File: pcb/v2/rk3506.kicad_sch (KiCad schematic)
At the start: 15 parts, among them J1 Conn_01x02, J2 Conn_01x03, J3 Conn_01x02, U1 SOM3562_18

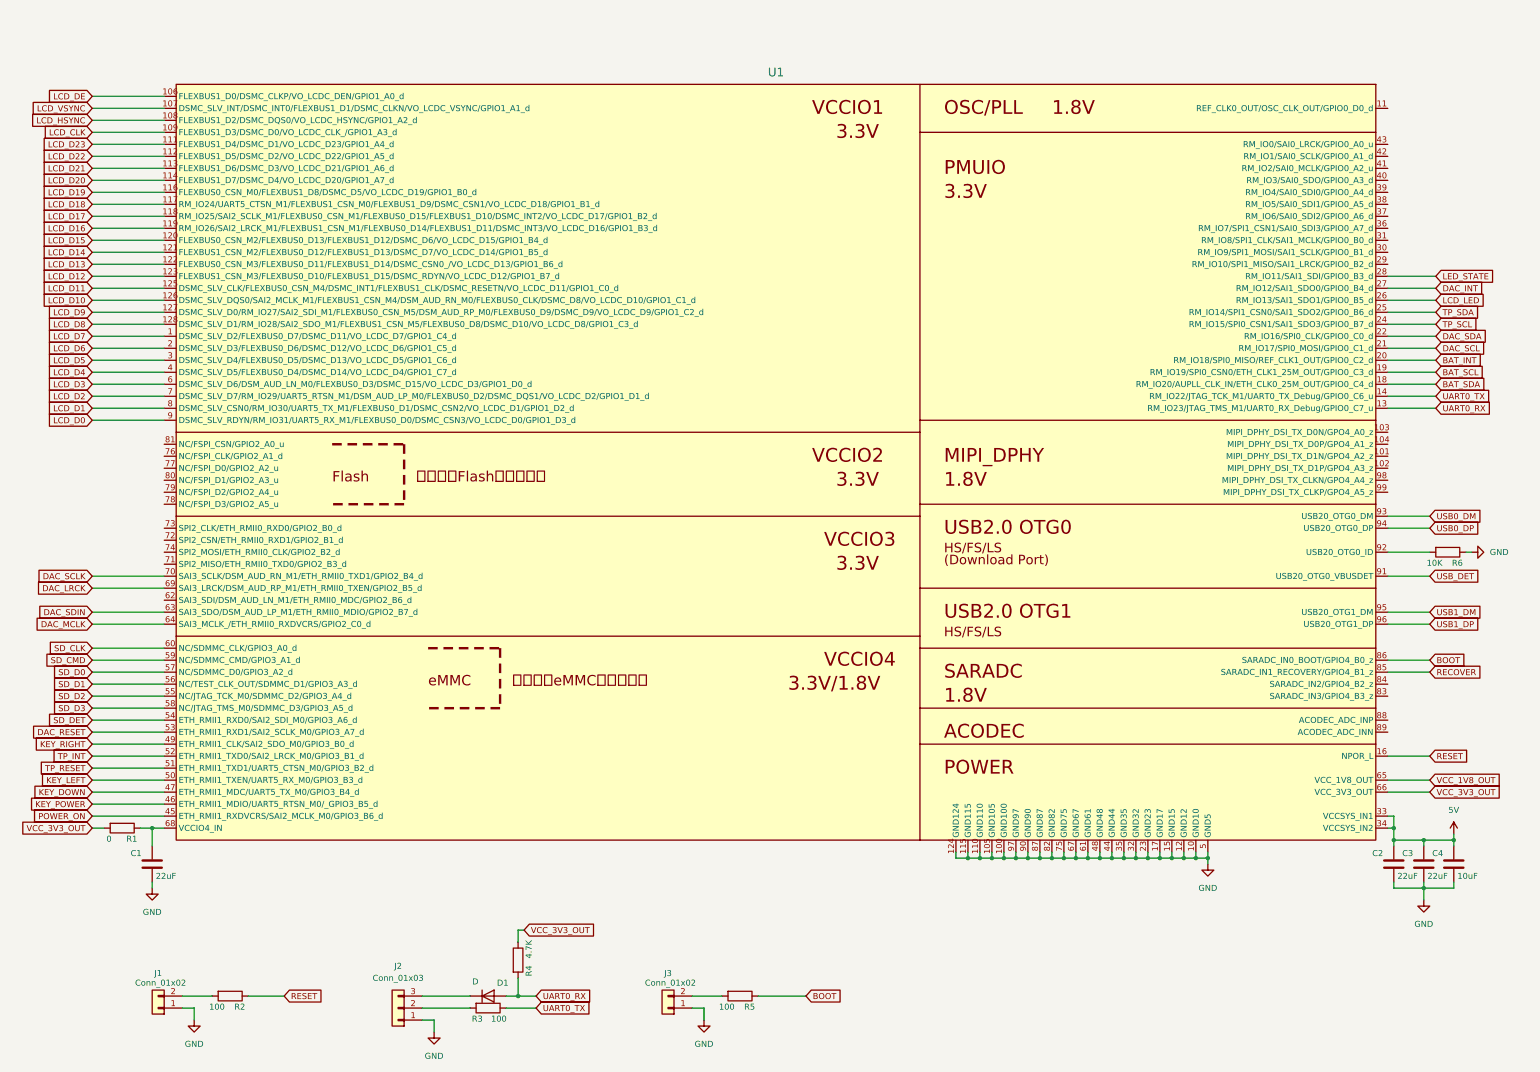
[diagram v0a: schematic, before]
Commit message: up fix lcd pcb
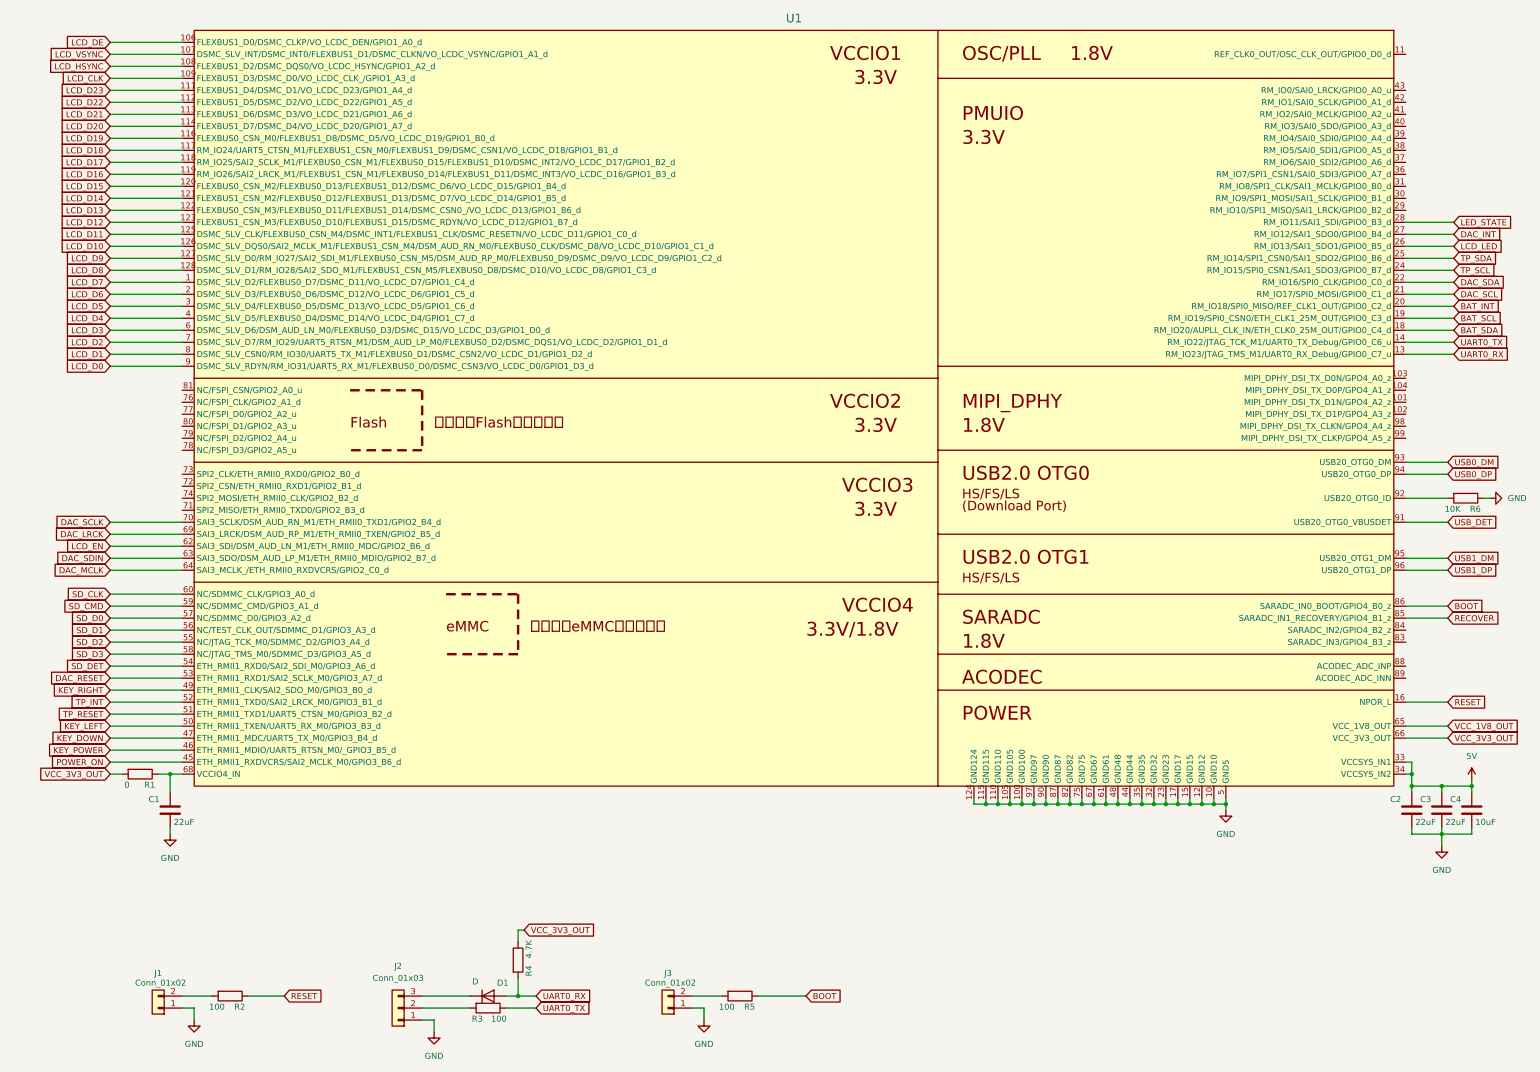
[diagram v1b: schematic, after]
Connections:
- net LCD_EN: now reaches U1.62 (SAI3_SDI/DSM_AUD_LN_M1/ETH_RMII0_MDC/GPIO2_B6_d)
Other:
- moved on the sheet: C1, C2, C3, C4, R1, R6, U1
